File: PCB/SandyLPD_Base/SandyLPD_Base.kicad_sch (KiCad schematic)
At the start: 232 parts, among them J1 Conn_02x02_Odd_Even, J10 Conn_01x10_Pin, J11 Conn_01x03, J2 Conn_01x03, J4 Conn_01x10_Pin, J5 USB_C_Receptacle_USB2.0, J6 USB_C_Receptacle_USB2.0, J7 USB_C_Receptacle_USB2.0, J8 USB_C_Receptacle_USB2.0, J9 Conn_02x02_Odd_Even, SW1 BOOT_ALT, SW2 RESET_ALT, SW3 SW_DIP_x04, SW4 BOOT_ALT, SW5 RESET_ALT, SW6 SW_DIP_x04, U1 NCP1117-3.3_SOT223, U2 NCP1117-3.3_SOT223, U3 RP2040, U4 W25Q128JVPIQ, U5 RP2040, U6 W25Q128JVPIQ, Y1 12MHz, Y2 12MHz

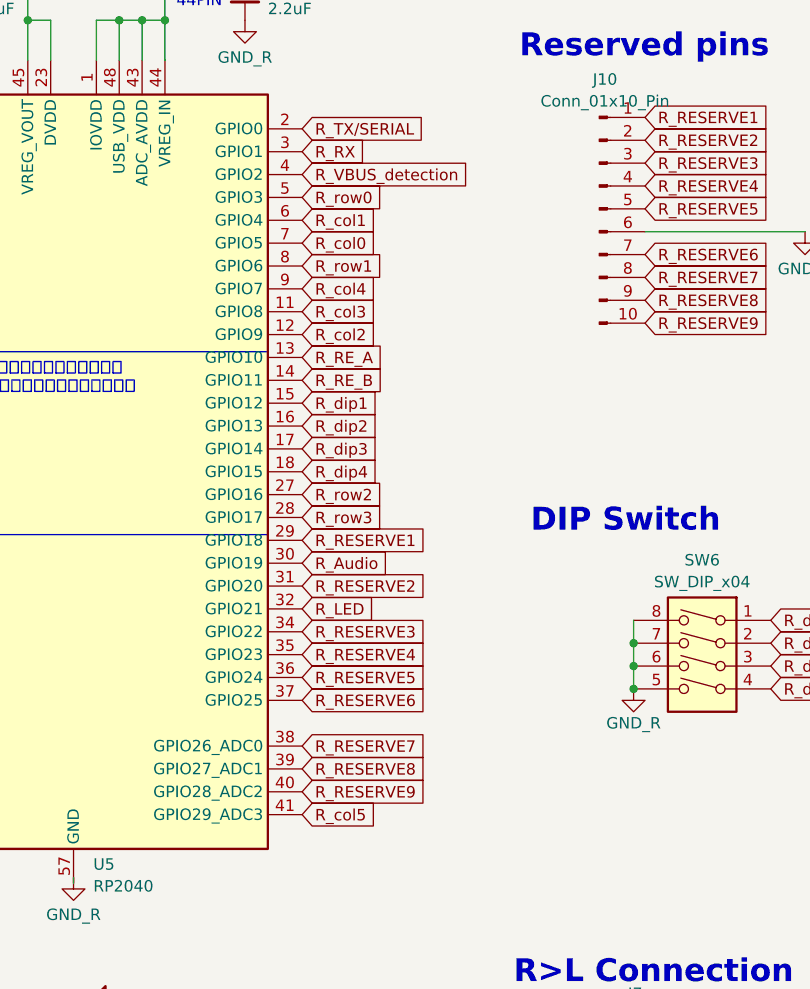
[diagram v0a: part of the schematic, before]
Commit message: 配線ひとまず完了
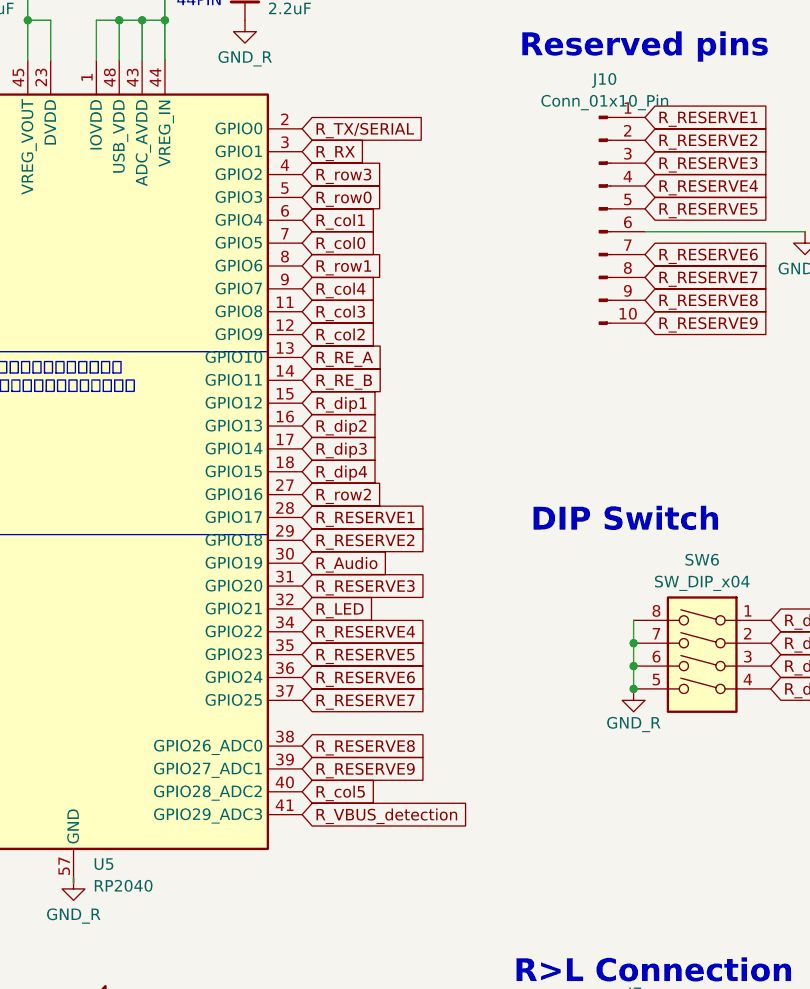
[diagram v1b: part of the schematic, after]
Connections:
- net R_RESERVE1: now also U5.28 (GPIO17); no longer U5.29 (GPIO18)
- net R_RESERVE2: now also U5.29 (GPIO18); no longer U5.31 (GPIO20)
- net R_RESERVE3: now also U5.31 (GPIO20); no longer U5.34 (GPIO22)
- net R_RESERVE4: now also U5.34 (GPIO22); no longer U5.35 (GPIO23)
- net R_RESERVE5: now also U5.35 (GPIO23); no longer U5.36 (GPIO24)
- net R_RESERVE6: now also U5.36 (GPIO24); no longer U5.37 (GPIO25)
- net R_RESERVE7: now also U5.37 (GPIO25); no longer U5.38 (GPIO26_ADC0)
- net R_RESERVE8: now also U5.38 (GPIO26_ADC0); no longer U5.39 (GPIO27_ADC1)
- net R_RESERVE9: now also U5.39 (GPIO27_ADC1); no longer U5.40 (GPIO28_ADC2)
- net R_VBUS_detection: now also U5.41 (GPIO29_ADC3); no longer U5.4 (GPIO2)
- net R_col5: now also U5.40 (GPIO28_ADC2); no longer U5.41 (GPIO29_ADC3)
- net R_row3: now also U5.4 (GPIO2); no longer U5.28 (GPIO17)
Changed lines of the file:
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@@
 	(global_label "R_RESERVE1"
 		(shape input)
-		(at 665.48 140.97 0)
+		(at 665.48 138.43 0)
 		(fields_autoplaced yes)
 		(effects
@@
 		)
 		(property "Intersheetrefs" "${INTERSHEET_REFS}"
-			(at 679.5432 140.97 0)
+			(at 679.5432 138.43 0)
 			(effects
 				(font
@@
 	(global_label "R_row3"
 		(shape input)
-		(at 665.48 138.43 0)
+		(at 665.48 100.33 0)
 		(fields_autoplaced yes)
 		(effects
@@
 		)
 		(property "Intersheetrefs" "${INTERSHEET_REFS}"
-			(at 674.5238 138.43 0)
+			(at 674.5238 100.33 0)
 			(effects
 				(font
@@
 		)
 		(property "シート間のリファレンス" "${INTERSHEET_REFS}"
-			(at 665.48 140.2652 0)
+			(at 665.48 102.1652 0)
 			(effects
 				(font
@@
 	(global_label "R_RESERVE7"
 		(shape input)
-		(at 665.48 163.83 0)
+		(at 665.48 158.75 0)
 		(fields_autoplaced yes)
 		(effects
@@
 		)
 		(property "Intersheetrefs" "${INTERSHEET_REFS}"
-			(at 679.5432 163.83 0)
+			(at 679.5432 158.75 0)
 			(effects
 				(font
@@
 	(global_label "R_RESERVE8"
 		(shape input)
-		(at 665.48 166.37 0)
+		(at 665.48 163.83 0)
 		(fields_autoplaced yes)
 		(effects
@@
 		)
 		(property "Intersheetrefs" "${INTERSHEET_REFS}"
-			(at 679.5432 166.37 0)
+			(at 679.5432 163.83 0)
 			(effects
 				(font
@@
 	(global_label "R_RESERVE5"
 		(shape input)
-		(at 665.48 156.21 0)
+		(at 665.48 153.67 0)
 		(fields_autoplaced yes)
 		(effects
@@
 		)
 		(property "Intersheetrefs" "${INTERSHEET_REFS}"
-			(at 679.5432 156.21 0)
+			(at 679.5432 153.67 0)
 			(effects
 				(font
@@
 	(global_label "R_RESERVE6"
 		(shape input)
-		(at 665.48 158.75 0)
+		(at 665.48 156.21 0)
 		(fields_autoplaced yes)
 		(effects
@@
 		)
 		(property "Intersheetrefs" "${INTERSHEET_REFS}"
-			(at 679.5432 158.75 0)
+			(at 679.5432 156.21 0)
 			(effects
 				(font
@@
 	(global_label "R_RESERVE4"
 		(shape input)
-		(at 665.48 153.67 0)
+		(at 665.48 151.13 0)
 		(fields_autoplaced yes)
 		(effects
@@
 		)
 		(property "Intersheetrefs" "${INTERSHEET_REFS}"
-			(at 679.5432 153.67 0)
+			(at 679.5432 151.13 0)
 			(effects
 				(font
@@
 	(global_label "R_RESERVE3"
 		(shape input)
-		(at 665.48 151.13 0)
+		(at 665.48 146.05 0)
 		(fields_autoplaced yes)
 		(effects
@@
 		)
 		(property "Intersheetrefs" "${INTERSHEET_REFS}"
-			(at 679.5432 151.13 0)
+			(at 679.5432 146.05 0)
 			(effects
 				(font
@@
 	(global_label "R_RESERVE2"
 		(shape input)
-		(at 665.48 146.05 0)
+		(at 665.48 140.97 0)
 		(fields_autoplaced yes)
 		(effects
@@
 		)
 		(property "Intersheetrefs" "${INTERSHEET_REFS}"
-			(at 679.5432 146.05 0)
+			(at 679.5432 140.97 0)
 			(effects
 				(font
@@
 	(global_label "R_RESERVE9"
 		(shape input)
-		(at 665.48 168.91 0)
+		(at 665.48 166.37 0)
 		(fields_autoplaced yes)
 		(effects
@@
 		)
 		(property "Intersheetrefs" "${INTERSHEET_REFS}"
-			(at 679.5432 168.91 0)
+			(at 679.5432 166.37 0)
 			(effects
 				(font
@@
 	(global_label "R_VBUS_detection"
 		(shape input)
-		(at 665.48 100.33 0)
+		(at 665.48 171.45 0)
 		(fields_autoplaced yes)
 		(effects
@@
 		)
 		(property "Intersheetrefs" "${INTERSHEET_REFS}"
-			(at 684.6838 100.33 0)
+			(at 684.6838 171.45 0)
 			(effects
 				(font
@@
 	(global_label "R_col5"
 		(shape input)
-		(at 665.48 171.45 0)
+		(at 665.48 168.91 0)
 		(fields_autoplaced yes)
 		(effects
@@
 		)
 		(property "Intersheetrefs" "${INTERSHEET_REFS}"
-			(at 674.1609 171.45 0)
+			(at 674.1609 168.91 0)
 			(effects
 				(font
@@
 		)
 		(property "シート間のリファレンス" "${INTERSHEET_REFS}"
-			(at 665.48 173.2852 0)
+			(at 665.48 170.7452 0)
 			(effects
 				(font
